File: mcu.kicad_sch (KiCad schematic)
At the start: 21 parts, among them J2 Conn_ARM_SWD_TagConnect_TC2030, SW1 SW_Push, U3 STM32L053R8Tx

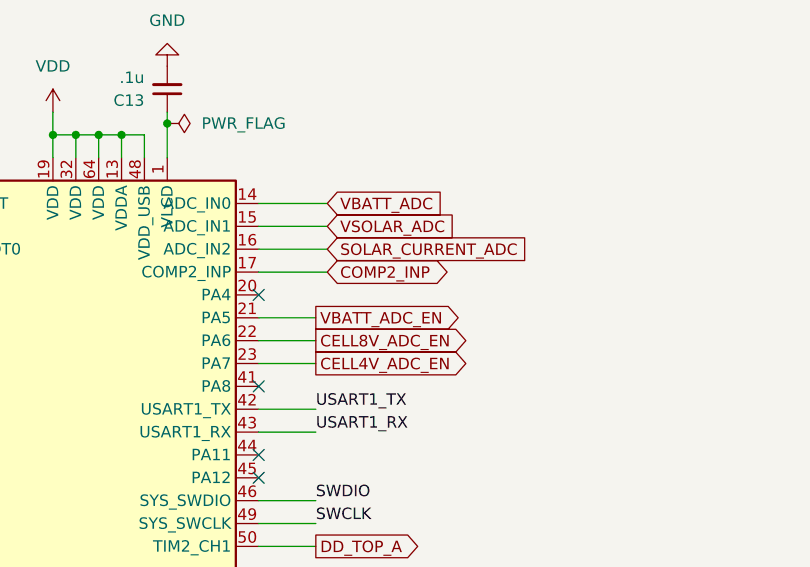
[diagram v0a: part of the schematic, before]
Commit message: 94 unrouted
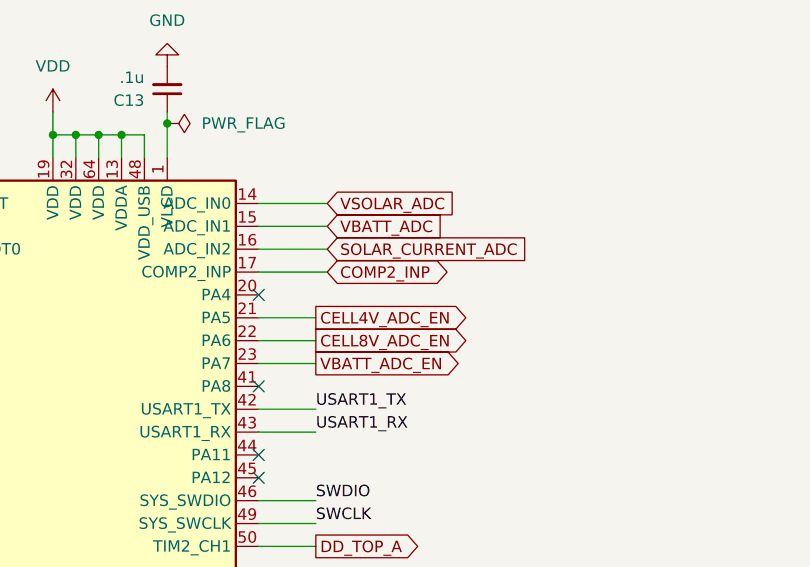
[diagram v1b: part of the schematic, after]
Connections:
- net CELL4V_ADC_EN: now also U3.21 (PA5); no longer U3.23 (PA7)
- net VBATT_ADC: now also U3.15 (PA1); no longer U3.14 (PA0)
- net VBATT_ADC_EN: now also U3.23 (PA7); no longer U3.21 (PA5)
- net VSOLAR_ADC: now also U3.14 (PA0); no longer U3.15 (PA1)
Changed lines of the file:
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@@
 	(global_label "VBATT_ADC"
 		(shape input)
-		(at 166.37 50.8 0)
+		(at 166.37 53.34 0)
 		(fields_autoplaced yes)
 		(effects
@@
 		)
 		(property "Intersheetrefs" "${INTERSHEET_REFS}"
-			(at 179.3338 50.8 0)
+			(at 179.3338 53.34 0)
 			(effects
 				(font
@@
 	(global_label "VSOLAR_ADC"
 		(shape input)
-		(at 166.37 53.34 0)
+		(at 166.37 50.8 0)
 		(fields_autoplaced yes)
 		(effects
@@
 		)
 		(property "Intersheetrefs" "${INTERSHEET_REFS}"
-			(at 180.9667 53.34 0)
+			(at 180.9667 50.8 0)
 			(effects
 				(font
@@
 	)
 	(global_label "CELL4V_ADC_EN"
+		(shape output)
+		(at 165.1 63.5 0)
+		(effects
+			(font
+				(size 1.27 1.27)
+			)
+			(justify left)
+		)
+		(property "Intersheetrefs" "${INTERSHEET_REFS}"
+			(at 165.1 63.5 0)
+			(effects
+				(font
+					(size 1.27 1.27)
+				)
+				(hide yes)
+			)
+		)
+	)
+	(global_label "VBATT_ADC_EN"
 		(shape output)
 		(at 165.1 68.58 0)
@@
 			(effects
 				(font
-					(size 1.27 1.27)
-				)
-				(hide yes)
-			)
-		)
-	)
-	(global_label "VBATT_ADC_EN"
-		(shape output)
-		(at 165.1 63.5 0)
-		(effects
-			(font
-				(size 1.27 1.27)
-			)
-			(justify left)
-		)
-		(property "Intersheetrefs" "${INTERSHEET_REFS}"
-			(at 165.1 63.5 0)
-			(effects
-				(font
